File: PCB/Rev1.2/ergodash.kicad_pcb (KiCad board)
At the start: 2 copper layers, 149.9 x 127.4 mm, 187 parts, among them J1 5PIN, J2 Conn_01x03, J3 Conn_01x03, J4 GS3, J5 GS3, M1 Speaker, Q1 IRLML6344TRPbF, SW1 SW_PUSH, SW10 SW_PUSH, SW11 SW_PUSH, SW12 SW_PUSH, SW13 SW_PUSH, SW14 SW_PUSH, SW15 SW_PUSH, SW16 SW_PUSH, SW17 SW_PUSH, SW18 SW_PUSH, SW19 SW_PUSH, SW2 SW_PUSH, SW20 SW_PUSH, SW21 SW_PUSH, SW22 SW_PUSH, SW23 SW_PUSH, SW24 SW_PUSH, SW25 SW_PUSH, SW26 SW_PUSH, SW27 SW_PUSH, SW28 SW_PUSH, SW29 SW_Push, SW3 SW_PUSH, SW30 SW_PUSH, SW31 SW_PUSH, SW32 SW_PUSH, SW33 SW_PUSH, SW34 SW_PUSH, SW35 SW_PUSH, SW36 SW_PUSH, SW37 SW_Push, SW38 SW_PUSH, SW39 SW_PUSH, SW4 SW_PUSH, SW40 SW_PUSH, SW41 SW_PUSH, SW5 SW_PUSH, SW6 SW_PUSH, SW7 SW_PUSH, SW8 SW_PUSH, SW9 SW_PUSH, U1 HOLE, U2 HOLE, U3 ProMicro, U4 HOLE, U5 HOLE, U6 ProMicro, U7 HOLE, U8 HOLE, U9 HOLE

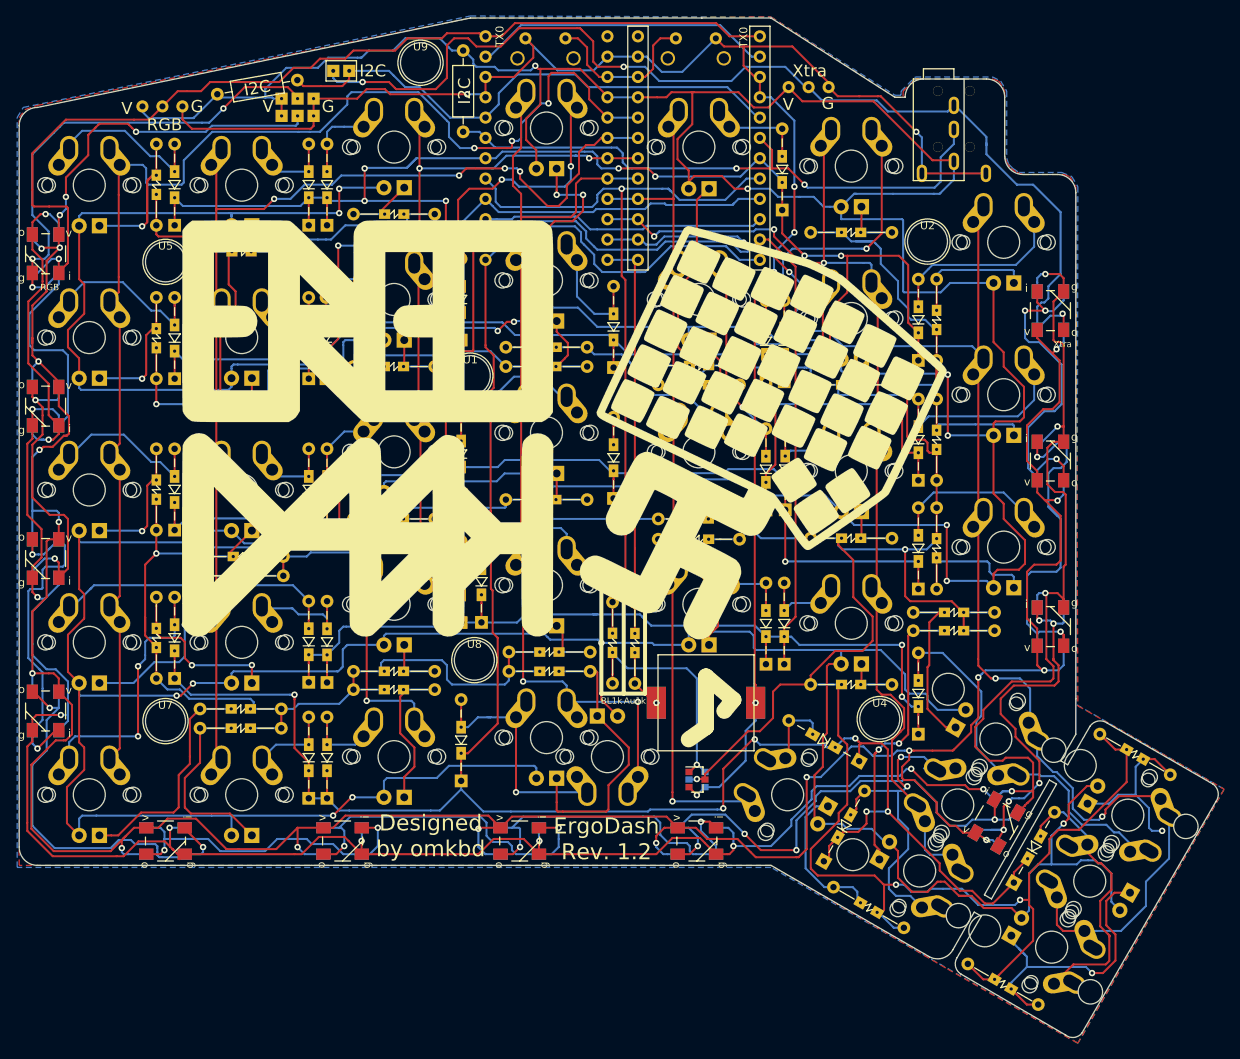
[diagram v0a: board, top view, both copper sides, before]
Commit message: Rev 1.2 project cleanup
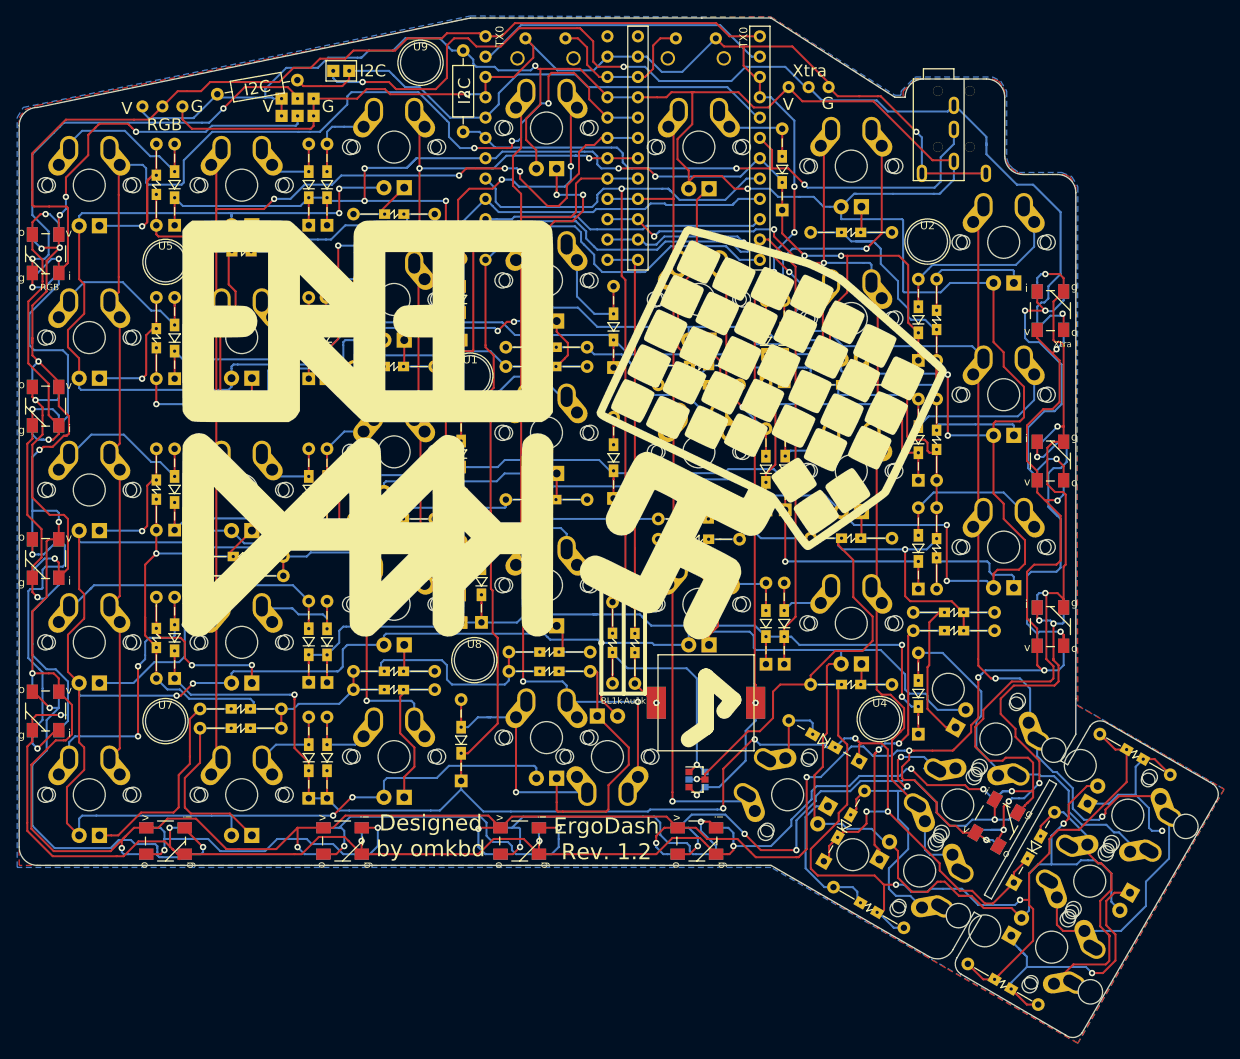
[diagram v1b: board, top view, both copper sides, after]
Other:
- net class Default removed
